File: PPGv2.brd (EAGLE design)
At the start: 46.2 x 35.8 mm, 54 parts

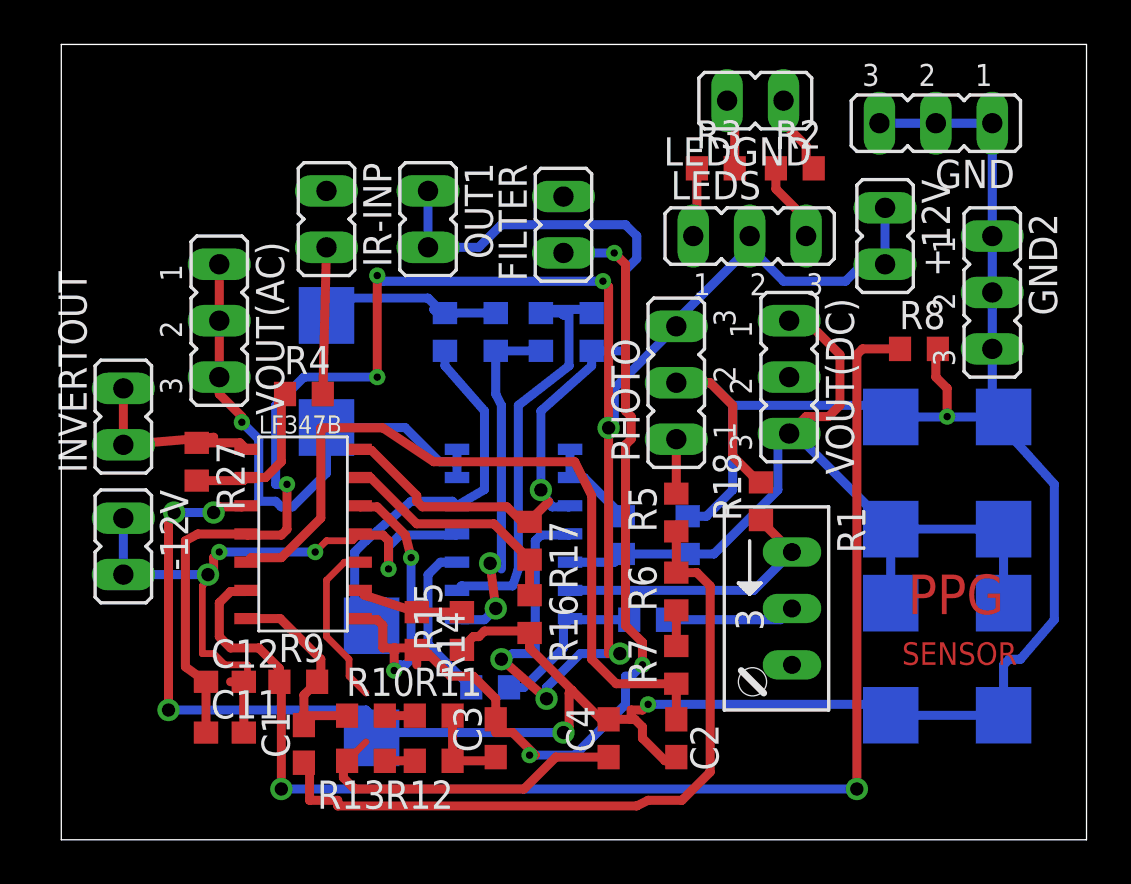
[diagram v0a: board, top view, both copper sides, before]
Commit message: Before removing the extra Pins
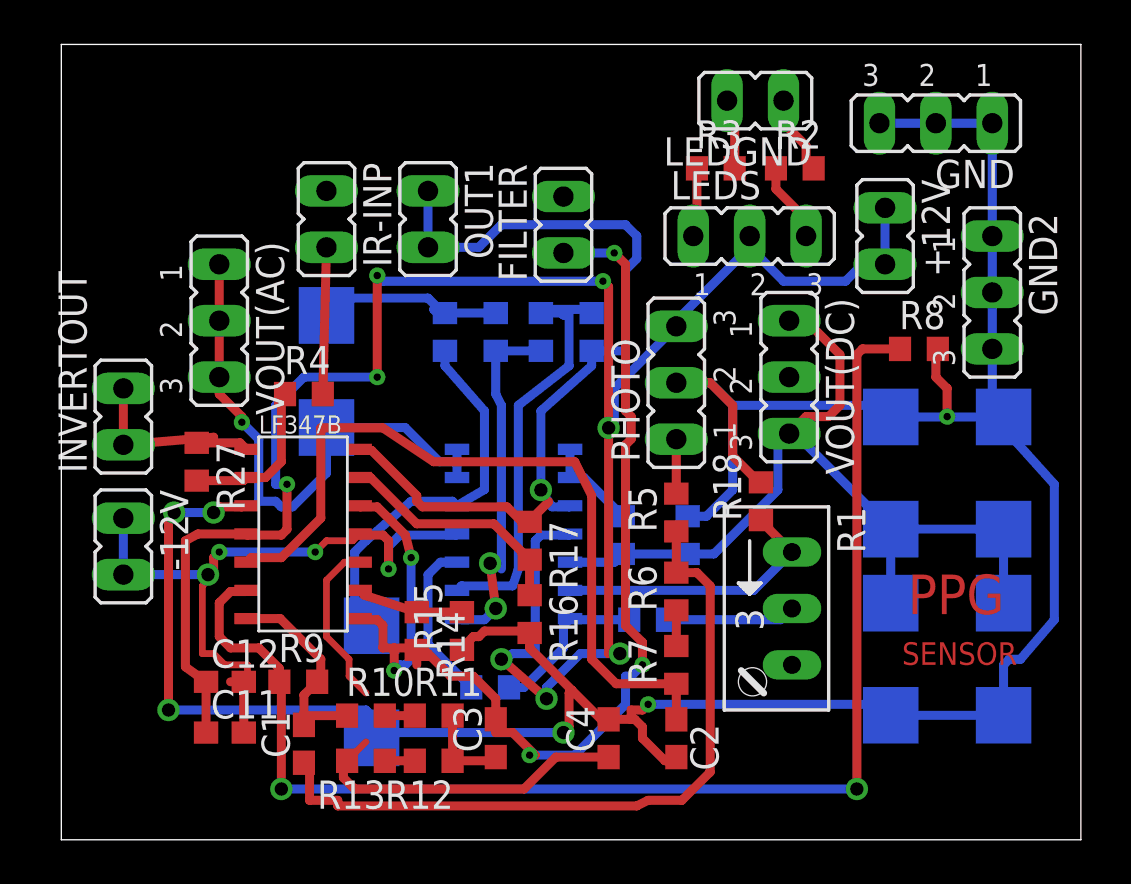
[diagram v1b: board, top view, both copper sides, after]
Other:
- board size 46.2 x 35.8 mm -> 45.9 x 35.8 mm
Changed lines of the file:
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@@
 <board>
 <plain>
-<wire x1="-29.21" y1="-24.638" x2="16.942" y2="-24.638" width="0" layer="20"/>
-<wire x1="16.942" y1="-24.638" x2="16.942" y2="11.166" width="0" layer="20"/>
-<wire x1="16.942" y1="11.166" x2="-29.21" y2="11.166" width="0" layer="20"/>
+<wire x1="-29.21" y1="-24.638" x2="16.688" y2="-24.638" width="0" layer="20"/>
+<wire x1="16.688" y1="-24.638" x2="16.688" y2="11.166" width="0" layer="20"/>
+<wire x1="16.688" y1="11.166" x2="-29.21" y2="11.166" width="0" layer="20"/>
 <wire x1="-29.21" y1="11.166" x2="-29.21" y2="-24.638" width="0" layer="20"/>
 <text x="8.89" y="-14.478" size="1.778" layer="1" font="vector">PPG</text>
